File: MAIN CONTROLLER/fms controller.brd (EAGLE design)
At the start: 145.3 x 80.3 mm, 60 parts, among them IC3 7805TV, IC5 7805TV, Q1 16MHz, T1 BC547, T2 BC547, T3 BC547, T4 BC547, T5 BC547, T6 BC547, T7 BC547, U1 328P

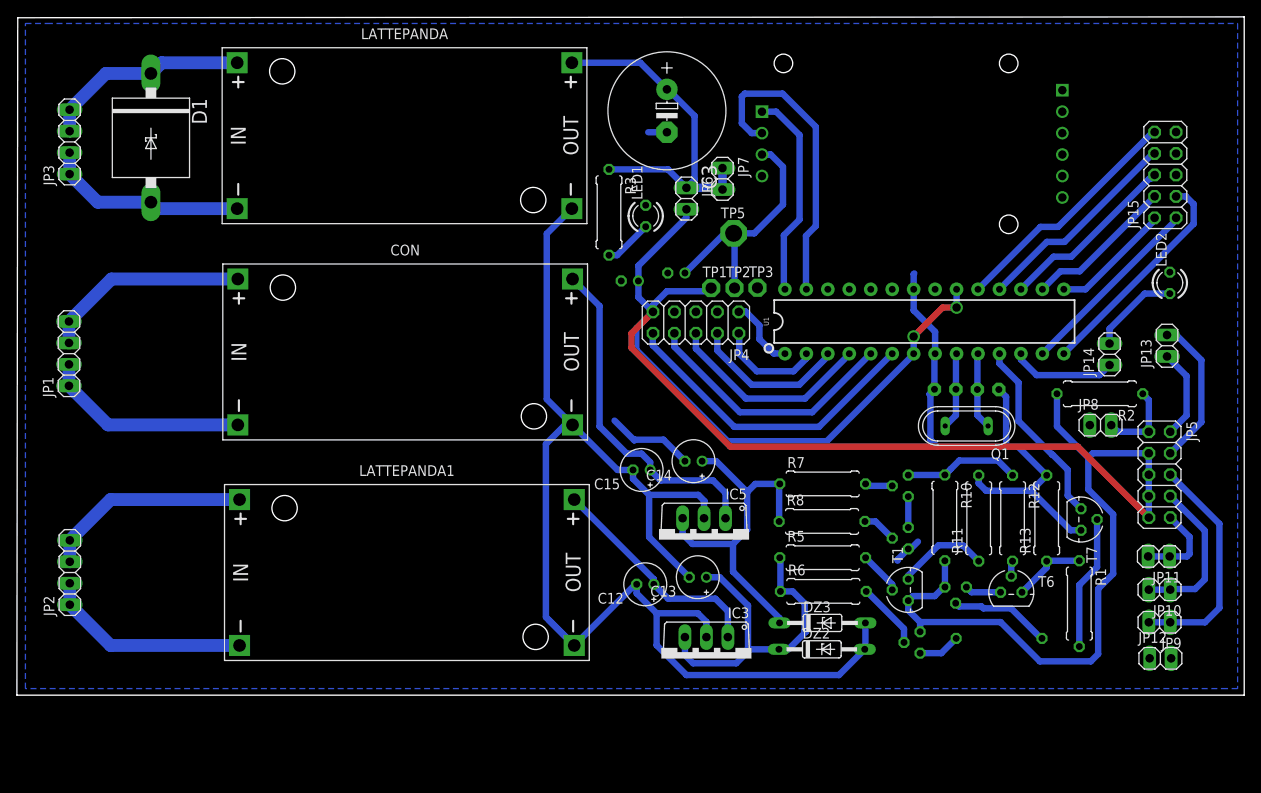
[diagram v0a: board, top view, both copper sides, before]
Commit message: 04/01/2020/08:38
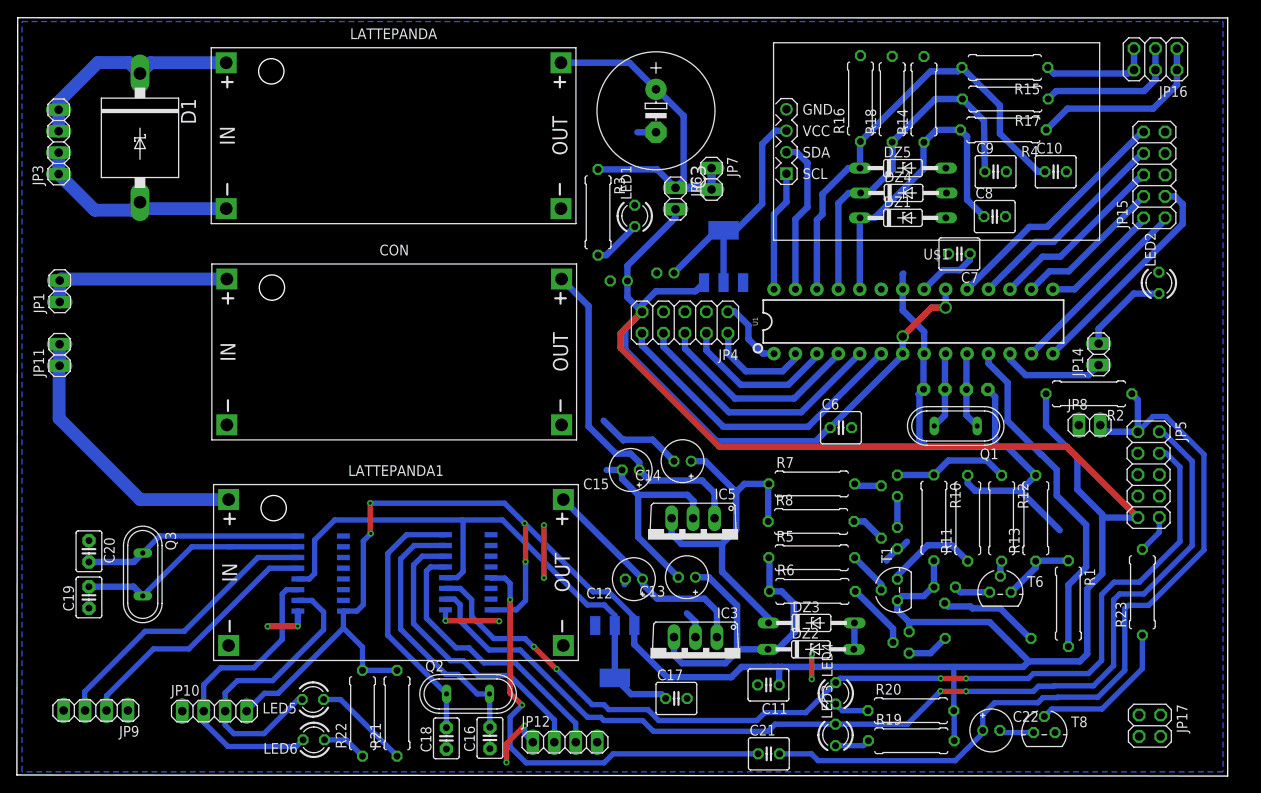
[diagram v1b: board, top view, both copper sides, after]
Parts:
- removed JP13: (no value), pinhead:1X02
- removed JP2: START, pinhead:1X04
- removed T7: BC547, transistor:TO92
- removed TP1, TP2, TP3: TPPAD1-13, testpad:P1-13
- removed TP5: TPPAD1-20, testpad:P1-20
- added C10, C11, C17, C21, C6, C7, C8, C9: 100nF, rcl:C025-040X050
- added C16, C18, C19, C20: 22pF, capacitor-wima:C2.5-3
- added C22: 10uF, rcl:E2-5
- added DZ1, DZ4, DZ5: 5.1, diode:DO35Z10
- added IC1, IC2: LM2936MP-3.3, national-semiconductor:SOT223
- added JP16: (no value), pinhead:2X03
- added JP17: (no value), pinhead:2X02
- added LED3, LED4, LED5, LED6: (no value), led:LED3MM
- added Q2, Q3: 12MHz, special:QS
- added R14, R16, R18: 100K, rcl:0309/10
- added R15, R17, R4: 1M, rcl:0309/10
- added R19, R20, R21, R22, R23: 1k, rcl:0309/10
- added T8: BC547, transistor:TO92
- added U$2, U$3: CH340G, ch340g:SOIC16
- C4: value 10uF -> 100uF
- JP1: value STOP -> (none); device pinhead:1X04 -> pinhead:1X02
- JP10, JP12, JP9: device pinhead:1X02 -> pinhead:1X04
- moved JP11 132.3 mm to (7.85, 57.3), turned to 90 degrees
- moved JP9 126.4 mm to (12.1, 15.2)
- moved JP10 112.8 mm to (26.2, 15.1), turned to 0 degrees
- moved JP12 71.2 mm to (67.7, 11.4)
- moved JP1 7.47 mm to (7.87, 64.8)
- moved U$1 2.91 mm to (111.7, 82.5), flipped to the top, turned to 180 degrees
- moved C12 1.48 mm to (75.8, 30.7)
- moved R1 1.30 mm to (127.3, 27.8)
- moved C1 1.30 mm to (111.4, 53.2)
- moved C13 1.30 mm to (82.1, 31.0)
- moved C14 1.30 mm to (81.6, 44.7)
- moved C15 1.30 mm to (75.5, 43.7)
- moved C2 1.30 mm to (116.5, 53.2)
- moved C3 1.30 mm to (78.5, 86.2)
- moved C4 1.30 mm to (74.1, 66.0)
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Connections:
- removed net GND.1: U$1.J1.6
- removed net N$2: R1.2, T7.2
- removed net N$4: CON.IN+, JP1.3, JP1.4
- removed net N$6: CON.IN-, JP1.1, JP1.2
- removed net VCC.1: U$1.J1.5
- new net ACCIN: JP16.1, JP16.2, R4.1
- new net ACCOUT: C8.1, DZ1.C, R14.1, R4.2, U1.24
- new net ALTIN: JP16.3, JP16.4, R17.1
- new net ALTOUT: C9.1, DZ4.C, R17.2, R18.1, U1.25
- new net D+MAIN: JP12.3, U$2.5
- new net D+RF: JP9.2, U$3.5
- new net D-MAIN: JP12.2, U$2.6
- new net D-RF: JP9.3, U$3.6
- new net DUMPIN: JP16.5, JP16.6, R15.1
- new net DUMPOUT: C10.1, DZ5.C, R15.2, R16.1, U1.26
- new net N$19: C7.1, U1.21
- new net N$20: C19.2, Q3.2, U$3.7
- new net N$22: C20.2, Q3.1, U$3.8
- new net N$23: C16.2, Q2.2, U$2.7
- new net N$28: C18.2, Q2.1, U$2.8
- new net N$31: C21.1, U$2.13
- new net N$33: C22.-, T8.3
- new net N$37: LED4.A, R20.1
- new net N$39: LED3.A, R19.1
- new net N$42: LED5.A, R21.1
- new net N$43: LED6.A, R22.1
- new net N$44: R23.1, T8.2
- new net RXRF: JP10.3, LED5.K, U$3.2
- new net TXRF: JP10.2, LED6.K, U$3.3
- new net VSS: C17.1, IC2.2, IC2.4, U$2.4, U$3.4
- net ACCEXT: no longer JP9.1, JP9.2
- net ALTEXT: no longer JP10.1, JP10.2
- net DUMPEXT: now also R23.2; no longer JP11.1, JP11.2
- net GND: now also C10.2, C11.2, C16.1, C17.2, C18.1, C19.1, C20.1, C6.2, C7.2, C8.2, C9.2, CON.IN-, DZ1.A, DZ4.A, DZ5.A, IC1.1, IC2.1, JP10.1, JP17.1, JP17.2, JP17.3, JP17.4, JP9.1, LATTEPANDA1.IN-, R14.2, R16.2, R18.2, T8.1, U$2.1, U$3.1; no longer JP12.2, T7.1, TP3.TP
- net LOAD: now also R1.2; no longer T7.3
- net N$1: now also JP11.1, JP11.2, LATTEPANDA1.IN+; no longer JP2.1, JP2.2, LATTEPANDA1.IN-
- net N$18: now also IC1.2, IC1.4; no longer TP2.TP, TP5.TP
- net N$3: now also CON.IN+, JP1.1, JP1.2; no longer JP2.3, JP2.4, LATTEPANDA1.IN+
- net RSTEXT: now also C21.2, C22.+
- net RXDEXT: now also LED3.K, U$2.2; no longer JP13.1
- net TXDEXT: now also LED4.K, U$2.3; no longer JP13.2
- net VCC: now also C11.1, C6.1, IC1.3, IC2.3, JP10.4, R19.2, R20.2, R21.2, R22.2, U$2.16, U$3.16; no longer JP5.3, JP5.5, JP5.7, TP1.TP
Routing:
- net VCC: track 284.7 -> 431.5 mm, vias 2 -> 6
- net RXDEXT: track 10.7 -> 125.0 mm, vias 0 -> 2
- net TXDEXT: track 17.8 -> 119.9 mm, vias 0 -> 4
- net GND: track 230.4 -> 140.4 mm, vias 0 -> 10
- net RSTEXT: track 9.60 -> 98.1 mm
- net VSS: track 0.00 -> 70.4 mm
- net N$31: track 0.00 -> 53.6 mm, vias 0 -> 2
- net DUMPOUT: track 0.00 -> 53.0 mm
- net ALTOUT: track 0.00 -> 41.6 mm
- net ACCOUT: track 0.00 -> 38.0 mm
- net TXRF: track 0.00 -> 37.1 mm
- net RXRF: track 0.00 -> 35.5 mm
- net D-MAIN: track 0.00 -> 35.2 mm
- net D-RF: track 0.00 -> 34.1 mm
- net D+MAIN: track 0.00 -> 33.1 mm
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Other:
- board size 145.3 x 80.3 mm -> 143.3 x 89.8 mm
